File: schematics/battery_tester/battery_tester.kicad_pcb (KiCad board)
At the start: 2 copper layers, 170 x 155 mm, 39 parts, among them J1 BATT1, J101 XIAO_LEFT, J102 XIAO_RIGHT, J103 ADS1115_1, J104 ADS1115_2, J105 LED_STRIP, J2 BATT2, J3 BATT3, J4 BATT4, J5 BATT5, J6 BATT6, J7 BATT7, J8 BATT8, Q1 IRLZ44N, Q2 IRLZ44N, Q3 IRLZ44N, Q4 IRLZ44N, Q5 IRLZ44N, Q6 IRLZ44N, Q7 IRLZ44N, Q8 IRLZ44N

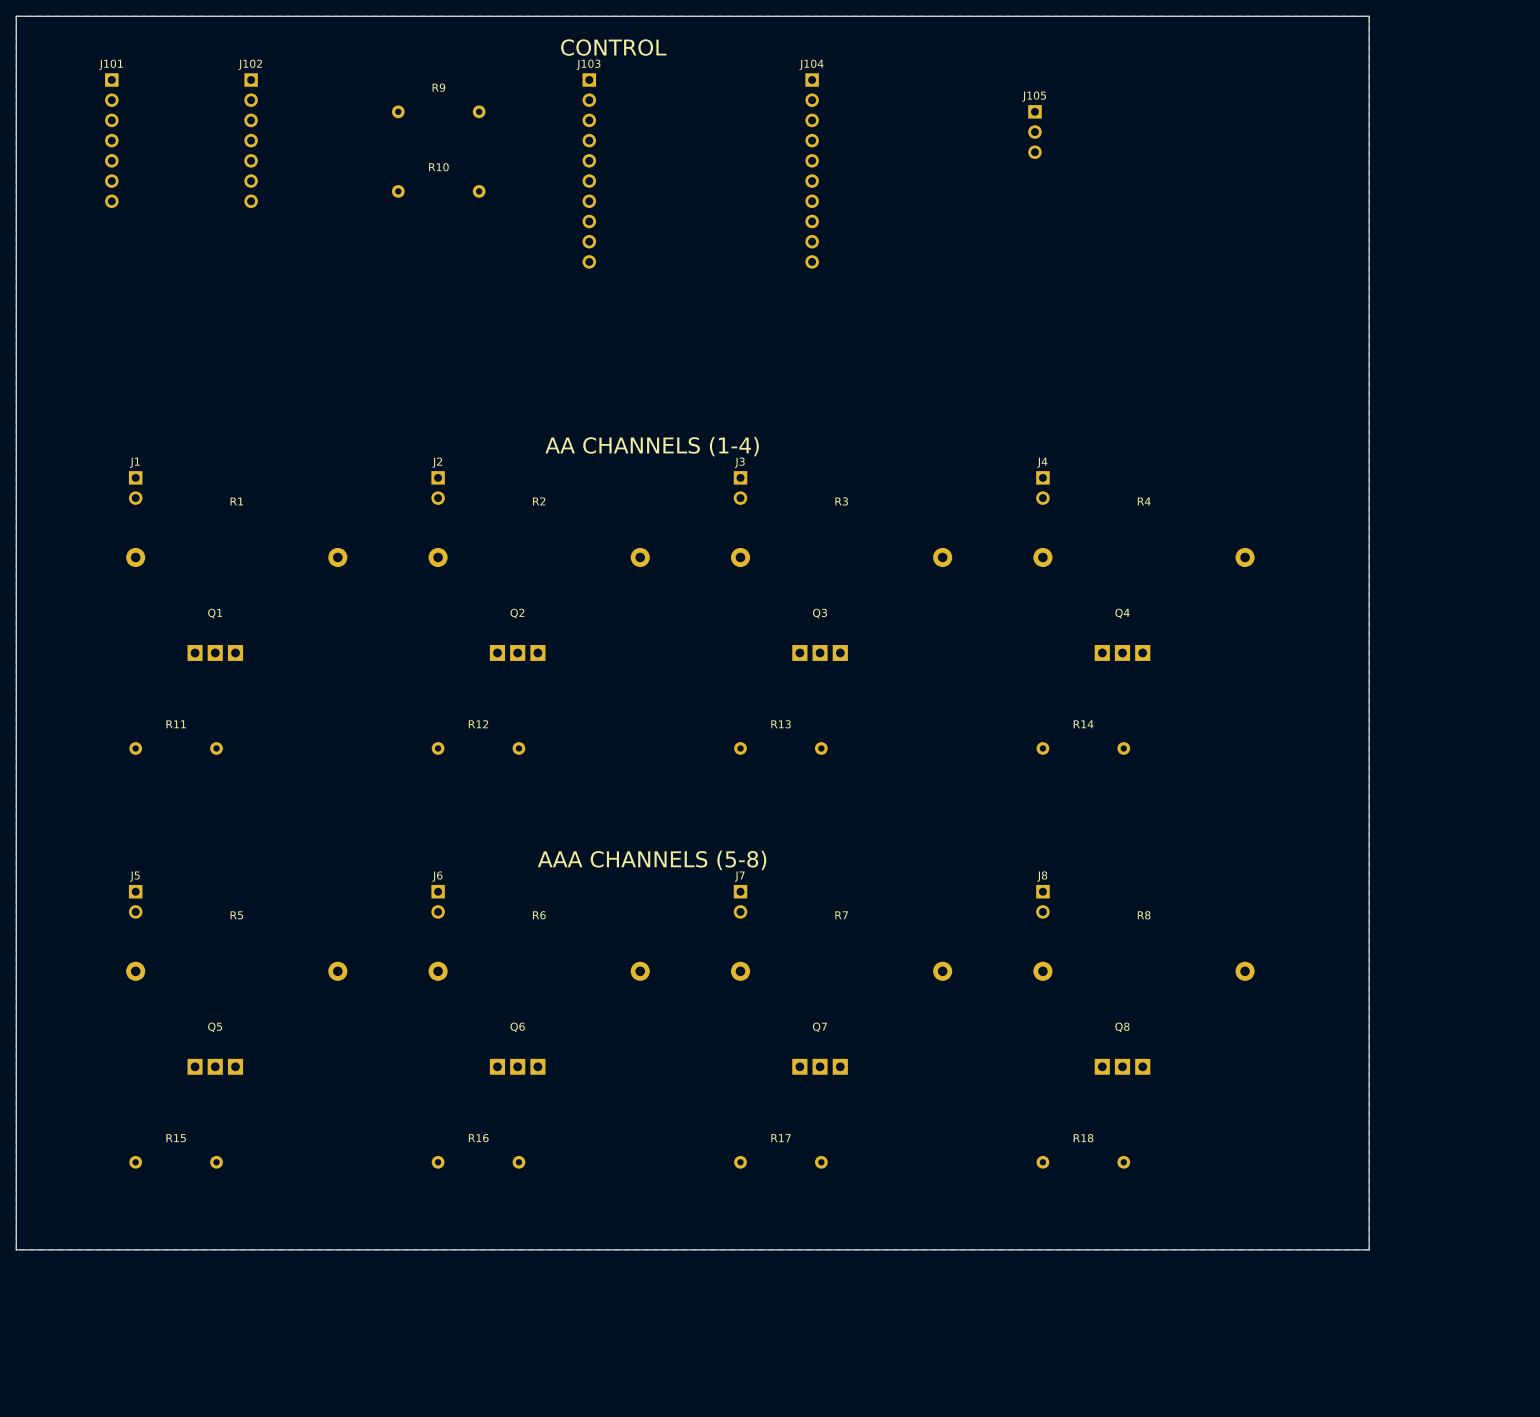
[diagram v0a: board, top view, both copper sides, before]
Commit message: Add v1.0.0 PCB layout with routed board and gerber outputs
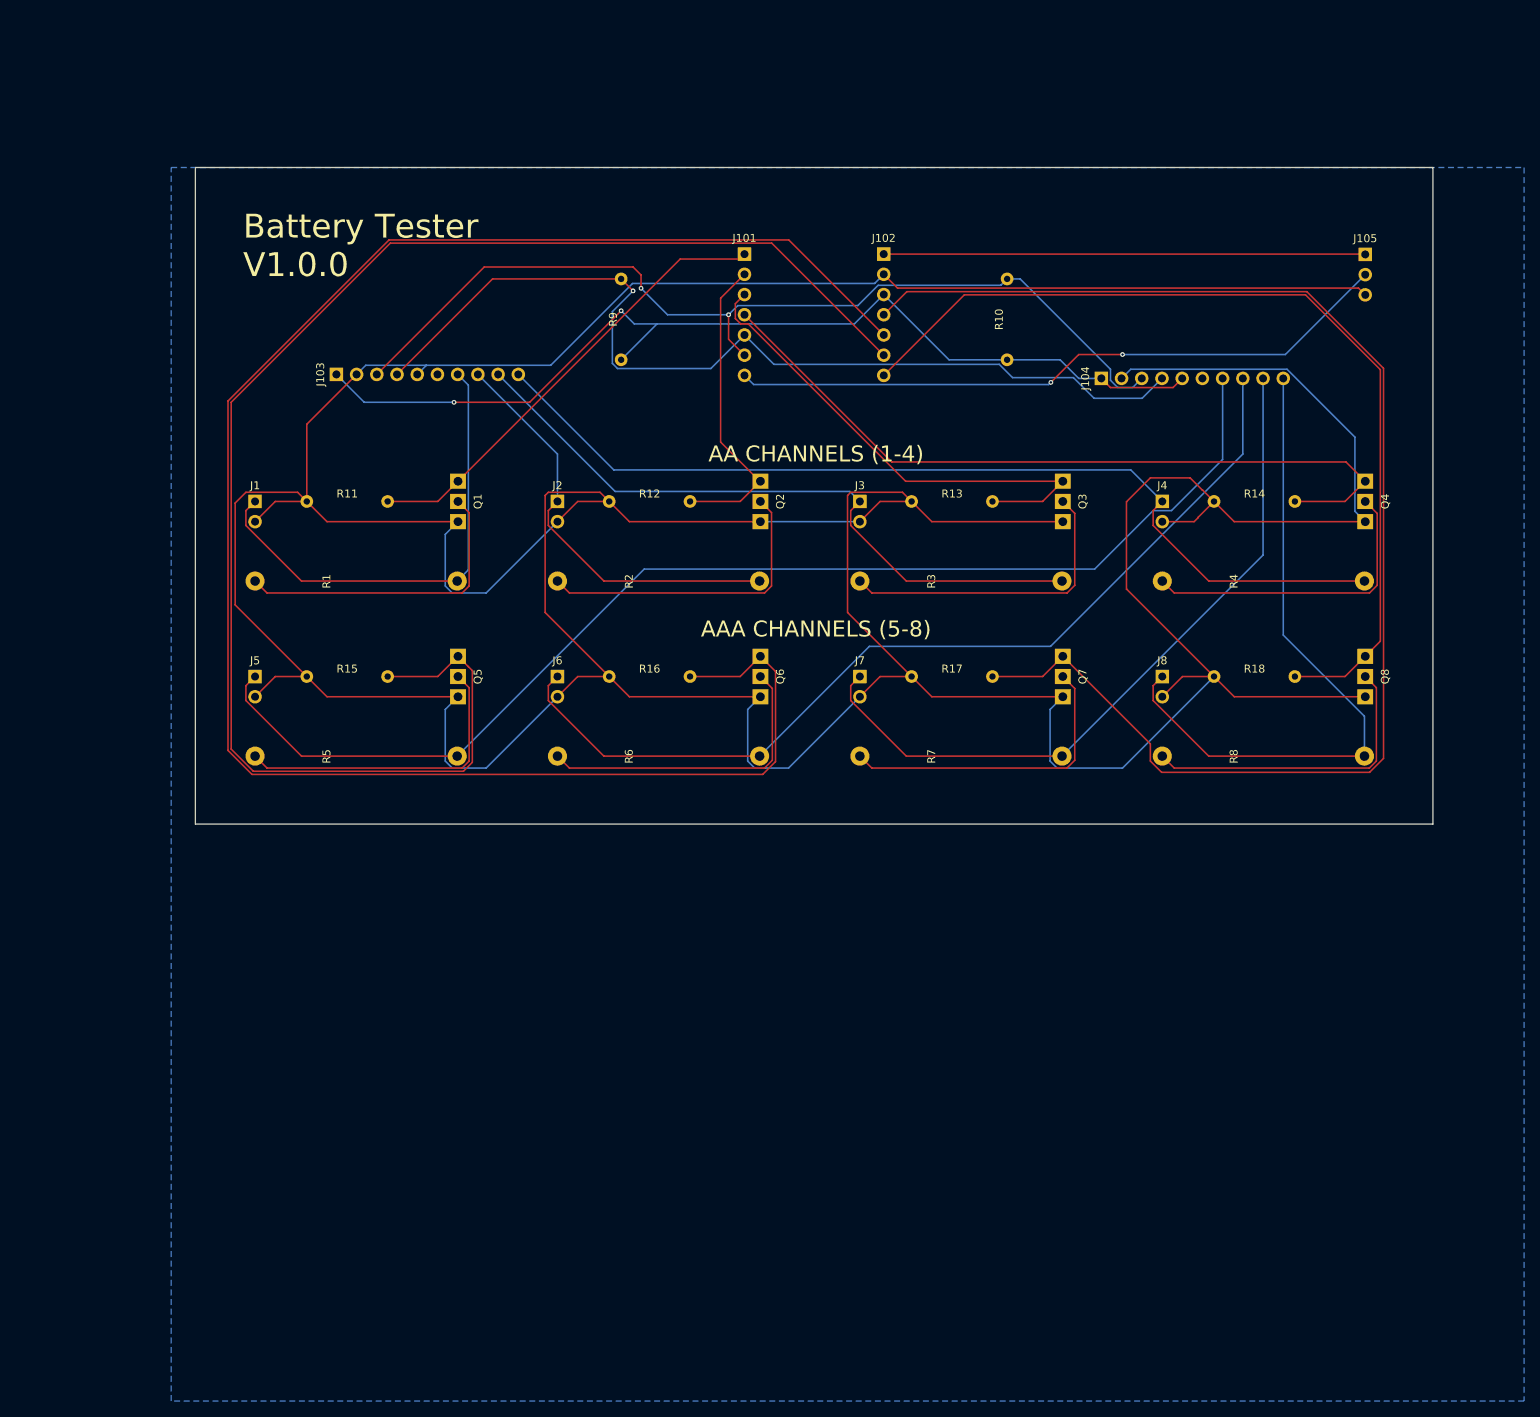
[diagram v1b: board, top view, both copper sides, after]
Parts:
- moved J101 82.5 mm to (91.5, 29.9)
- moved J102 82.5 mm to (109.0, 29.9)
- moved R10 77.3 mm to (124.5, 33.0), turned to -90 degrees
- moved R15 64.7 mm to (36.5, 83.0)
- moved R16 64.7 mm to (74.5, 83.0)
- moved R17 64.7 mm to (112.5, 83.0)
- moved R18 64.7 mm to (150.5, 83.0)
- moved Q5 57.8 mm to (55.5, 83.0), turned to -90 degrees
- moved Q6 57.8 mm to (93.5, 83.0), turned to -90 degrees
- moved Q7 57.8 mm to (131.5, 83.0), turned to -90 degrees
- moved Q8 57.8 mm to (169.5, 83.0), turned to -90 degrees
- moved J104 52.2 mm to (136.3, 45.5), turned to 90 degrees
- moved J103 48.8 mm to (40.2, 45.0), turned to 90 degrees
- moved J105 45.2 mm to (169.5, 29.9)
- moved R11 37.8 mm to (36.5, 61.0)
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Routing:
- net GND: track 0.00 -> 691.6 mm
- net GPIO9: track 0.00 -> 234.3 mm
- net GPIO8: track 0.00 -> 195.6 mm
- net GPIO10: track 0.00 -> 175.2 mm
- net BATT5+: track 0.00 -> 154.7 mm
- net +3V3: track 0.00 -> 126.4 mm, vias 0 -> 2
- net SDA: track 0.00 -> 120.9 mm, vias 0 -> 1
- net BATT4+: track 0.00 -> 120.5 mm
- net SCL: track 0.00 -> 119.9 mm, vias 0 -> 2
- net BATT6+: track 0.00 -> 118.9 mm
- net GPIO20: track 0.00 -> 117.2 mm
- net GPIO5: track 0.00 -> 96.6 mm
- net BATT7+: track 0.00 -> 90.9 mm
- net BATT3+: track 0.00 -> 85.0 mm
- net BATT8+: track 0.00 -> 84.6 mm
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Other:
- board size 170 x 155 mm -> 155.5 x 82.5 mm
- board text added: "Battery Tester V1.0.0"
- board text removed: "CONTROL"
